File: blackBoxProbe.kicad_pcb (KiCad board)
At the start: 4 copper layers, 44 x 44 mm, 81 parts, among them J1 USB-ID, J2 JTAG_2X05, J3 JTAG_2X05, J4 Conn_01x04, Q1 Q_NMOS_DUAL, Q2 Q_PMOS_DUAL, U1 MCP1702-MB, U2 USBLC6-2, U3 STM32F103CBT, U4 74X2T45, U5 74X2T45, U6 74X2T45, U7 74X2T45, Y1 Crystal

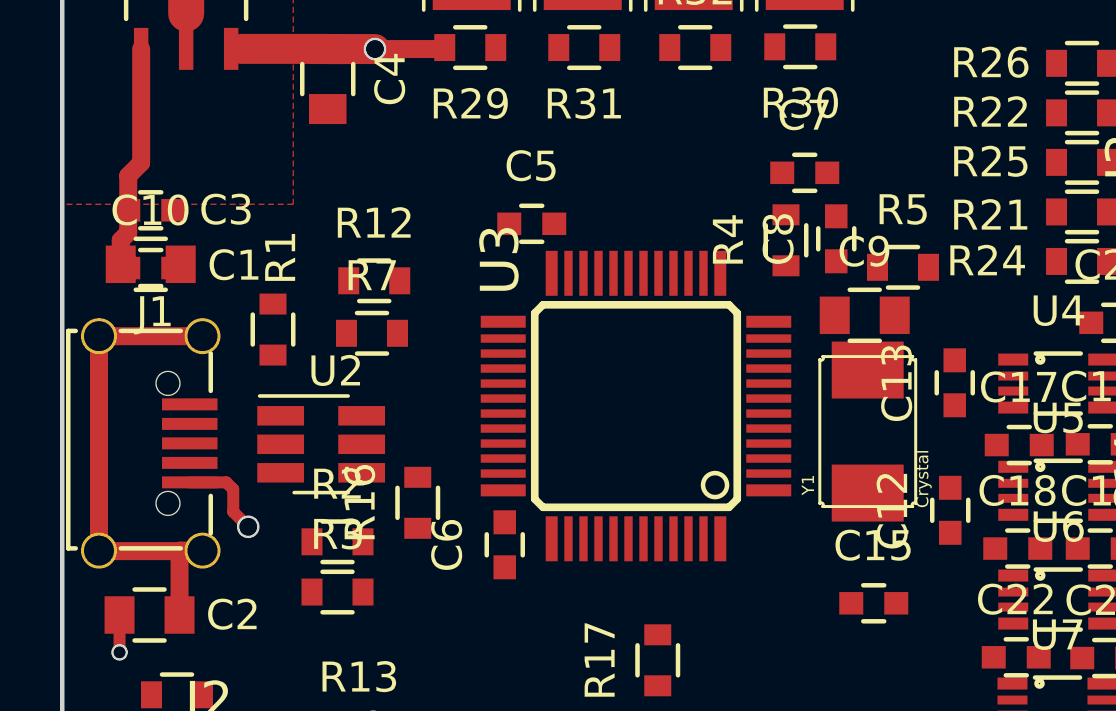
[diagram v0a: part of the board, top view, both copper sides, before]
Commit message: DONE: netlist updates
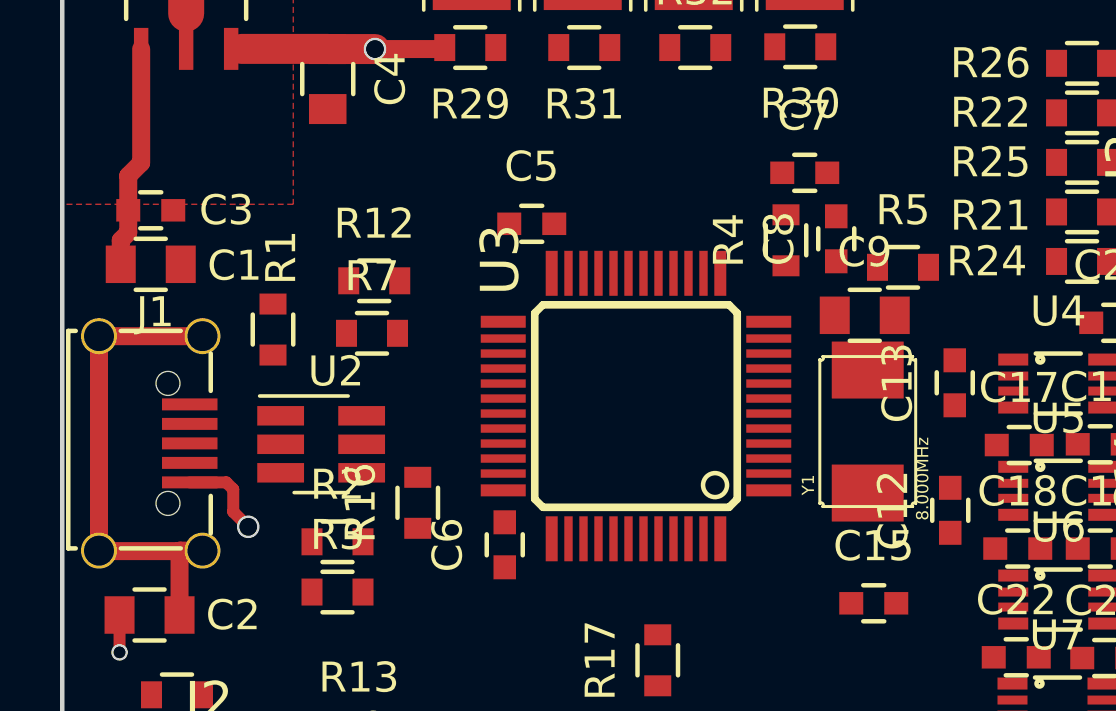
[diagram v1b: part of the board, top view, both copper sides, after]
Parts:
- removed C10: 100n, SquantorRcl:C_0603
- Y1: value Crystal -> 8.000MHz
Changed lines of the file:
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@@
 (kicad_pcb (version 4) (host pcbnew 4.0.7-e2-6376~61~ubuntu18.04.1)
   (general
-    (links 187)
-    (no_connects 186)
-    (area 14.147999 84.682 199.190187 197.252)
+    (links 185)
+    (no_connects 174)
+    (area 14.224999 151.174999 58.375001 195.325001)
     (thickness 1.6)
     (drawings 10)
     (tracks 27)
     (zones 0)
-    (modules 81)
+    (modules 80)
     (nets 76)
   )
@@
   )
   (module SquantorRcl:C_0603 (layer F.Cu)
-    (at 17.25 165.125)
-    (descr "Capacitor SMD 0603, reflow soldering, AVX (see smccp.pdf)")
-    (tags "capacitor 0603")
-    (attr smd)
-    (fp_text reference C10 (at 0 -1.9) (layer F.SilkS)
-      (effects (font (size 1 1) (thickness 0.15)))
-    )
-    (fp_text value 100n (at 0 1.9) (layer F.Fab)
-      (effects (font (size 1 1) (thickness 0.15)))
-    )
-    (fp_line (start -0.8 0.4) (end -0.8 -0.4) (layer F.Fab) (width 0.15))
-    (fp_line (start 0.8 0.4) (end -0.8 0.4) (layer F.Fab) (width 0.15))
-    (fp_line (start 0.8 -0.4) (end 0.8 0.4) (layer F.Fab) (width 0.15))
-    (fp_line (start -0.8 -0.4) (end 0.8 -0.4) (layer F.Fab) (width 0.15))
-    (fp_line (start -1.45 -0.75) (end 1.45 -0.75) (layer F.CrtYd) (width 0.05))
-    (fp_line (start -1.45 0.75) (end 1.45 0.75) (layer F.CrtYd) (width 0.05))
-    (fp_line (start -1.45 -0.75) (end -1.45 0.75) (layer F.CrtYd) (width 0.05))
-    (fp_line (start 1.45 -0.75) (end 1.45 0.75) (layer F.CrtYd) (width 0.05))
-    (fp_line (start -0.35 -0.6) (end 0.35 -0.6) (layer F.SilkS) (width 0.15))
-    (fp_line (start 0.35 0.6) (end -0.35 0.6) (layer F.SilkS) (width 0.15))
-    (pad 1 smd rect (at -0.75 0) (size 0.8 0.75) (layers F.Cu F.Paste F.Mask)
-      (net 1 +5V))
-    (pad 2 smd rect (at 0.75 0) (size 0.8 0.75) (layers F.Cu F.Paste F.Mask)
-      (net 2 GND))
-    (model Capacitors_SMD.3dshapes/C_0603.wrl
-      (at (xyz 0 0 0))
-      (scale (xyz 1 1 1))
-      (rotate (xyz 0 0 0))
-    )
-  )
-  (module SquantorRcl:C_0603 (layer F.Cu)
     (at 56.125 171.05 90)
     (descr "Capacitor SMD 0603, reflow soldering, AVX (see smccp.pdf)")
@@
       (effects (font (size 0.4064 0.4064) (thickness 0.0254)))
     )
-    (fp_text value Crystal (at -1.5748 1.8288 90) (layer F.SilkS)
+    (fp_text value 8.000MHz (at -1.5748 1.8288 90) (layer F.SilkS)
       (effects (font (size 0.4064 0.4064) (thickness 0.0254)))
     )
